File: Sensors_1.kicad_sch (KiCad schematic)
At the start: 25 parts, among them J7 Conn_01x04_Pin, J8 Conn_01x06_Pin, J9 Conn_01x02_Pin, U3 Ai-Thinker-Ra-01

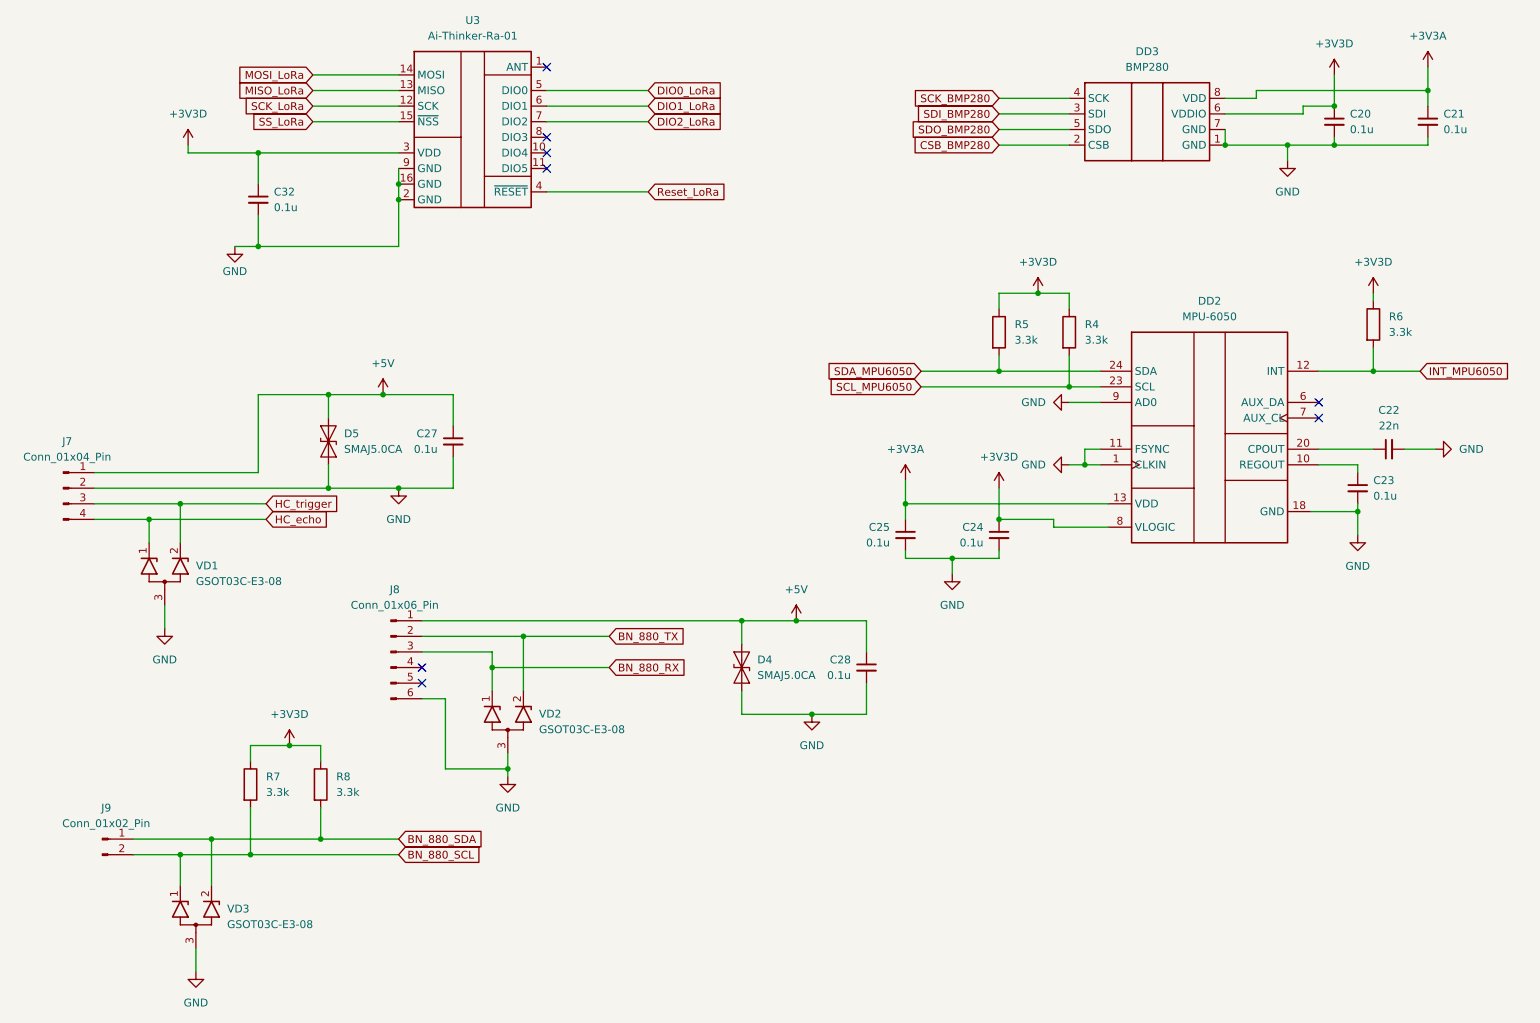
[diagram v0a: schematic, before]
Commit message: feat: Добавил внешние интерфейсы
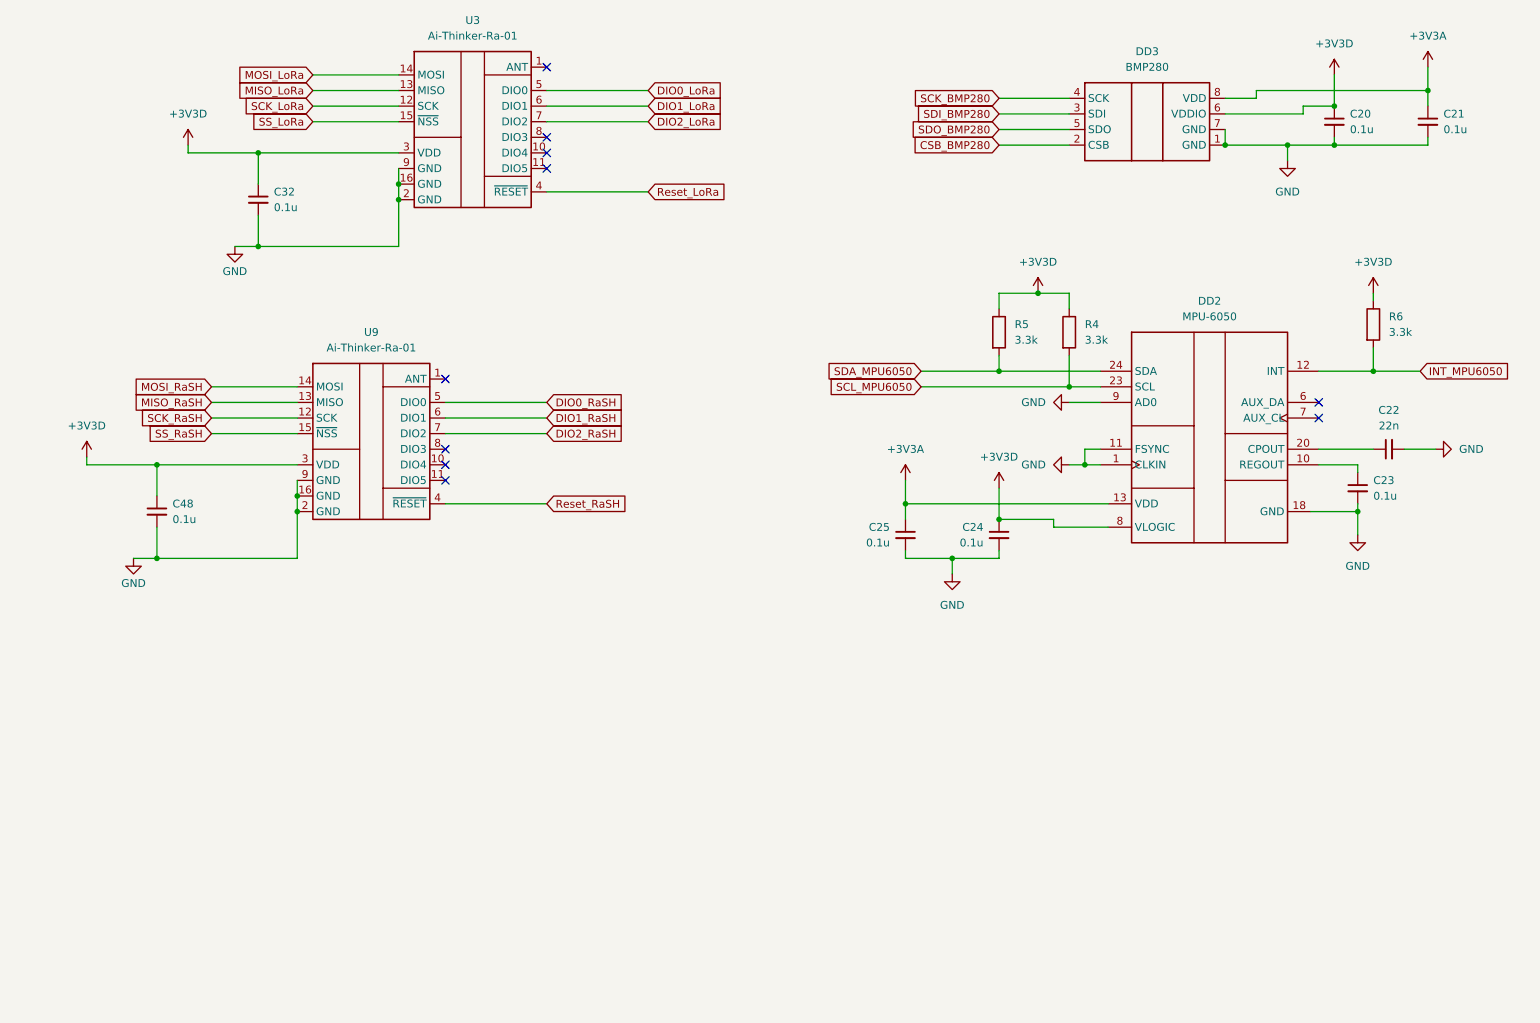
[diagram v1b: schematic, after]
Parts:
- removed C27, C28: 0.1u, Capacitor_SMD:C_0805_2012Metric_Pad1.18x1.45mm_HandSolder, symbol Device:C_Small
- removed D4, D5: SMAJ5.0CA, Diode_SMD:D_SMA, symbol Diode:SMAJ5.0CA
- removed J7: Conn_01x04_Pin, Connector_PinHeader_2.54mm:PinHeader_1x04_P2.54mm_Horizontal, symbol Connector:Conn_01x04_Pin
- removed J8: Conn_01x06_Pin, Connector_Hirose:Hirose_DF13-06P-1.25DSA_1x06_P1.25mm_Vertical, symbol Connector:Conn_01x06_Pin
- removed J9: Conn_01x02_Pin, Connector_Hirose:Hirose_DF13-02P-1.25DSA_1x02_P1.25mm_Vertical, symbol Connector:Conn_01x02_Pin
- removed R7, R8: 3.3k, Resistor_SMD:R_0805_2012Metric_Pad1.20x1.40mm_HandSolder, symbol Device:R
- removed VD1, VD2, VD3: GSOT03C-E3-08, Package_TO_SOT_SMD:SOT-23_Handsoldering, symbol TWS:GSOT03C-E3-08
- added C48: 0.1u, Capacitor_SMD:C_0805_2012Metric_Pad1.18x1.45mm_HandSolder, symbol Device:C_Small
- added U9: Ai-Thinker-Ra-01, RF_Module:Ai-Thinker-Ra-01-LoRa, symbol Receiver_and_transmitter:Ai-Thinker-Ra-01
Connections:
- net +3V3D: now also C48.1, U9.3 (VDD)
- net GND: now also C48.2, U9.16 (GND), U9.2 (GND), U9.9 (GND)
- new net DIO0_RaSH: U9.5 (DIO0)
- new net DIO1_RaSH: U9.6 (DIO1)
- new net DIO2_RaSH: U9.7 (DIO2)
- new net MISO_RaSH: U9.13 (MISO)
- new net MOSI_RaSH: U9.14 (MOSI)
- new net Reset_RaSH: U9.4 (~{RESET})
- new net SCK_RaSH: U9.12 (SCK)
- new net SS_RaSH: U9.15 (~{NSS})
- no-connect marks 8 -> 10
